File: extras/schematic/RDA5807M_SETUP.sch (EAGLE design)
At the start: 8 parts, among them Q1 32768k

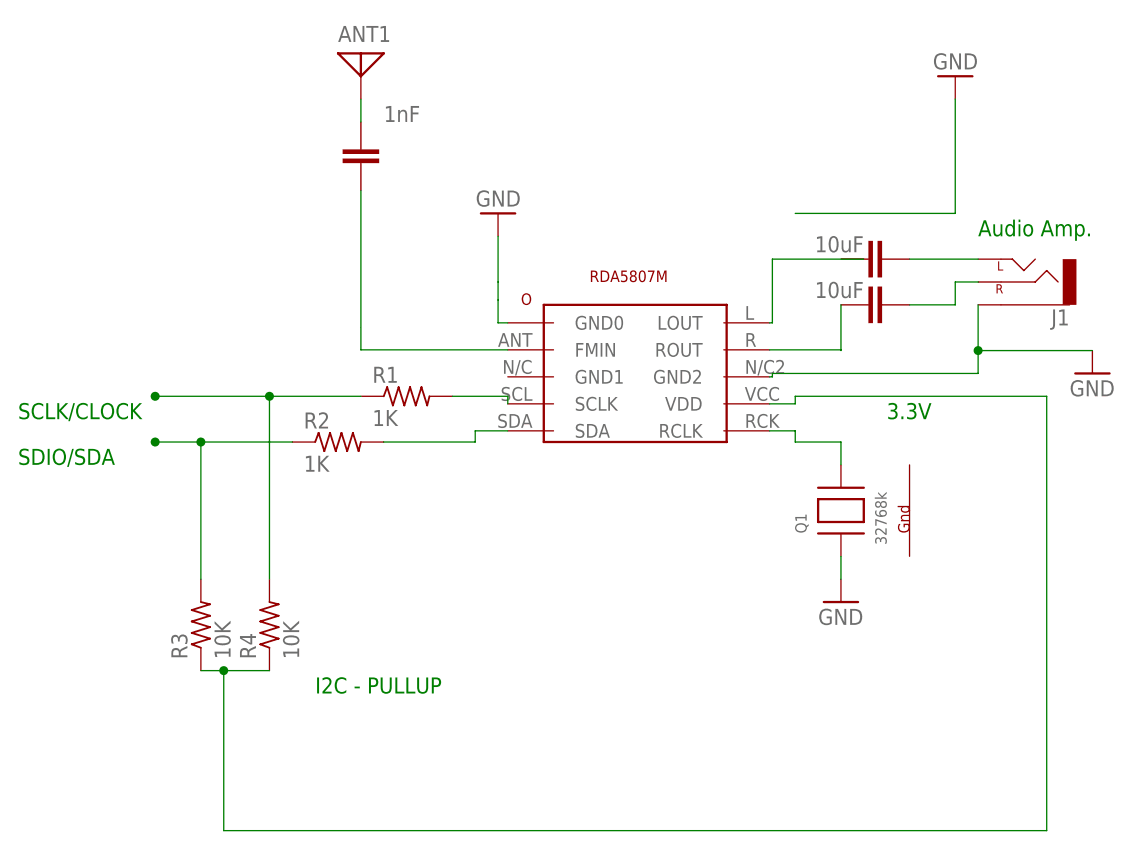
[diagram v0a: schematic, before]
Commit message: Extras
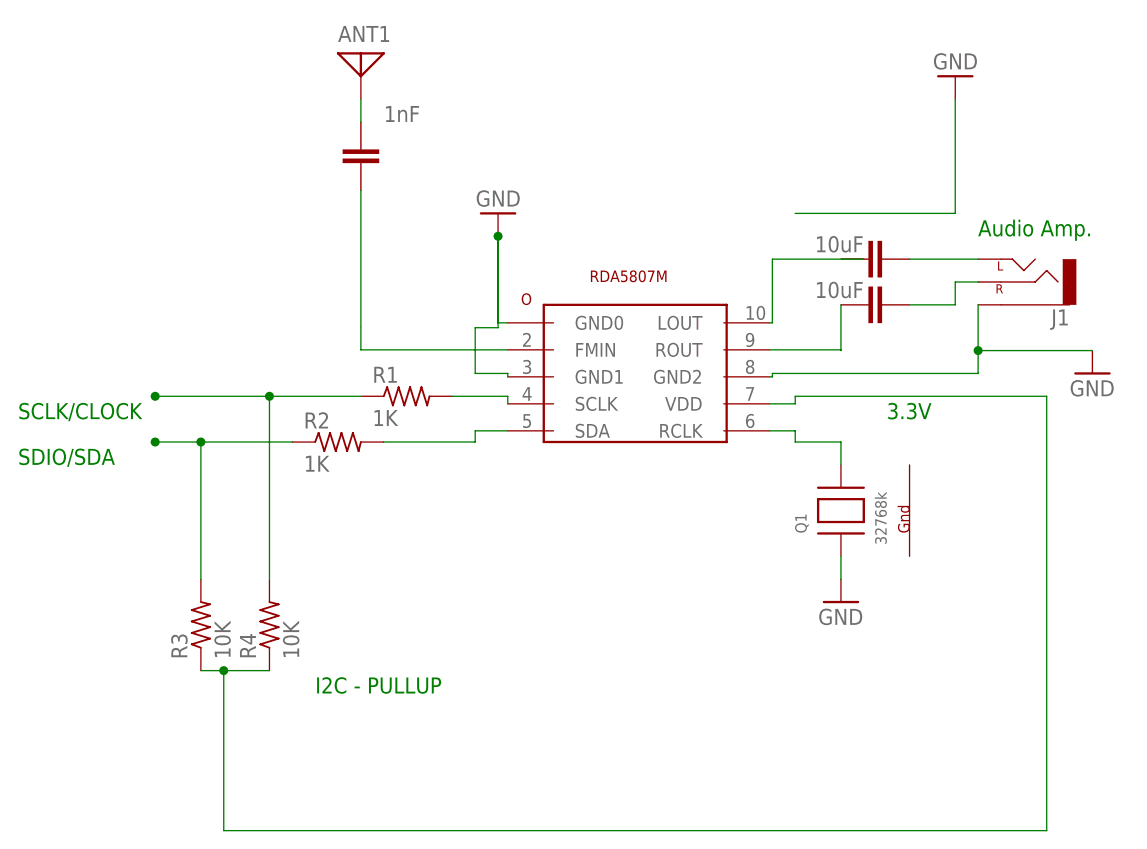
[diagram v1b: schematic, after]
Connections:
- removed net GND0: U$1.GND0
- new net GND1: U$1.GND0, U$1.GND1
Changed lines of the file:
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@@
 <segment>
 <pinref part="R1" gate="G$1" pin="2"/>
-<pinref part="U$1" gate="G$1" pin="SCLK"/>
 <wire x1="120.46" y1="16.94" x2="120.46" y2="17.78" width="0.1524" layer="91"/>
 <wire x1="120.46" y1="17.78" x2="114.3" y2="17.78" width="0.1524" layer="91"/>
+<pinref part="U$1" gate="G$1" pin="SCLK"/>
 </segment>
 </net>
@@
 <pinref part="R2" gate="G$1" pin="2"/>
 <wire x1="106.68" y1="12.7" x2="116.84" y2="12.7" width="0.1524" layer="91"/>
-<pinref part="U$1" gate="G$1" pin="SDA"/>
 <wire x1="120.46" y1="13.94" x2="116.84" y2="13.94" width="0.1524" layer="91"/>
 <wire x1="116.84" y1="13.94" x2="116.84" y2="12.7" width="0.1524" layer="91"/>
+<pinref part="U$1" gate="G$1" pin="SDA"/>
 </segment>
 </net>
@@
 <segment>
 <wire x1="149.86" y1="33.02" x2="160.02" y2="33.02" width="0.1524" layer="91"/>
-<pinref part="U$1" gate="G$1" pin="LOUT"/>
 <wire x1="149.54" y1="25.94" x2="149.86" y2="25.94" width="0.1524" layer="91"/>
 <wire x1="149.86" y1="25.94" x2="149.86" y2="33.02" width="0.1524" layer="91"/>
+<pinref part="U$1" gate="G$1" pin="LOUT"/>
 </segment>
 </net>
 <net name="N$7" class="0">
 <segment>
-<pinref part="U$1" gate="G$1" pin="ROUT"/>
 <wire x1="149.54" y1="22.94" x2="157.48" y2="22.94" width="0.1524" layer="91"/>
 <wire x1="157.48" y1="22.94" x2="157.48" y2="22.86" width="0.1524" layer="91"/>
 <wire x1="157.48" y1="22.94" x2="157.48" y2="27.94" width="0.1524" layer="91"/>
+<pinref part="U$1" gate="G$1" pin="ROUT"/>
 </segment>
 </net>
@@
 <wire x1="152.4" y1="12.7" x2="157.48" y2="12.7" width="0.1524" layer="91"/>
 <wire x1="157.48" y1="12.7" x2="157.48" y2="10.16" width="0.1524" layer="91"/>
-<pinref part="U$1" gate="G$1" pin="RCLK"/>
 <wire x1="149.54" y1="13.94" x2="152.4" y2="13.94" width="0.1524" layer="91"/>
 <wire x1="152.4" y1="13.94" x2="152.4" y2="12.7" width="0.1524" layer="91"/>
+<pinref part="U$1" gate="G$1" pin="RCLK"/>
 </segment>
 </net>
@@
 <wire x1="180.34" y1="-30.48" x2="180.34" y2="17.78" width="0.1524" layer="91"/>
 <wire x1="180.34" y1="17.78" x2="152.4" y2="17.78" width="0.1524" layer="91"/>
-<pinref part="U$1" gate="G$1" pin="VDD"/>
 <wire x1="149.54" y1="16.94" x2="152.4" y2="16.94" width="0.1524" layer="91"/>
 <wire x1="152.4" y1="16.94" x2="152.4" y2="17.78" width="0.1524" layer="91"/>
+<pinref part="U$1" gate="G$1" pin="VDD"/>
 </segment>
 </net>
@@
 </segment>
 </net>
-<net name="GND0" class="0">
-<segment>
-<pinref part="GND2" gate="1" pin="GND"/>
-<wire x1="119.38" y1="28.48" x2="119.38" y2="30.48" width="0.1524" layer="91"/>
-<pinref part="U$1" gate="G$1" pin="GND0"/>
-<wire x1="119.38" y1="30.48" x2="119.38" y2="35.56" width="0.1524" layer="91"/>
-<wire x1="120.46" y1="25.94" x2="119.38" y2="25.94" width="0.1524" layer="91"/>
-<wire x1="119.38" y1="25.94" x2="119.38" y2="28.48" width="0.1524" layer="91"/>
-</segment>
-</net>
 <net name="N$11" class="0">
 <segment>
-<pinref part="U$1" gate="G$1" pin="FMIN"/>
 <wire x1="120.46" y1="22.94" x2="104.14" y2="22.94" width="0.1524" layer="91"/>
 <wire x1="104.14" y1="22.94" x2="104.14" y2="25.4" width="0.1524" layer="91"/>
+<pinref part="U$1" gate="G$1" pin="FMIN"/>
 </segment>
 </net>
 <net name="GND2" class="0">
 <segment>
-<pinref part="U$1" gate="G$1" pin="GND2"/>
 <wire x1="149.54" y1="19.94" x2="149.86" y2="19.94" width="0.1524" layer="91"/>
 <wire x1="149.86" y1="19.94" x2="149.86" y2="20.32" width="0.1524" layer="91"/>
@@
 <wire x1="172.72" y1="20.32" x2="172.72" y2="22.86" width="0.1524" layer="91"/>
 <junction x="172.72" y="22.86"/>
+<pinref part="U$1" gate="G$1" pin="GND2"/>
 </segment>
 </net>
+<net name="GND1" class="0">
+<segment>
+<pinref part="U$1" gate="G$1" pin="GND1"/>
+<wire x1="120.46" y1="19.94" x2="120.46" y2="20.32" width="0.1524" layer="91"/>
+<wire x1="120.46" y1="20.32" x2="116.84" y2="20.32" width="0.1524" layer="91"/>
+<wire x1="116.84" y1="20.32" x2="116.84" y2="25.4" width="0.1524" layer="91"/>
+<wire x1="116.84" y1="25.4" x2="119.38" y2="25.4" width="0.1524" layer="91"/>
+<pinref part="GND2" gate="1" pin="GND"/>
+<wire x1="119.38" y1="25.94" x2="119.38" y2="35.56" width="0.1524" layer="91"/>
+<wire x1="120.46" y1="25.94" x2="119.38" y2="25.94" width="0.1524" layer="91"/>
+<pinref part="U$1" gate="G$1" pin="GND0"/>
+<wire x1="119.38" y1="25.4" x2="119.38" y2="35.56" width="0.1524" layer="91"/>
+<junction x="119.38" y="35.56"/>
+</segment>
+</net>
